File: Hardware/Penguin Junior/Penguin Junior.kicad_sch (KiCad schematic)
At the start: 30 parts, among them SW1 SW_Push, SW2 SW_SPDT, U1 STM32F405RGTx, Y1 16MHz

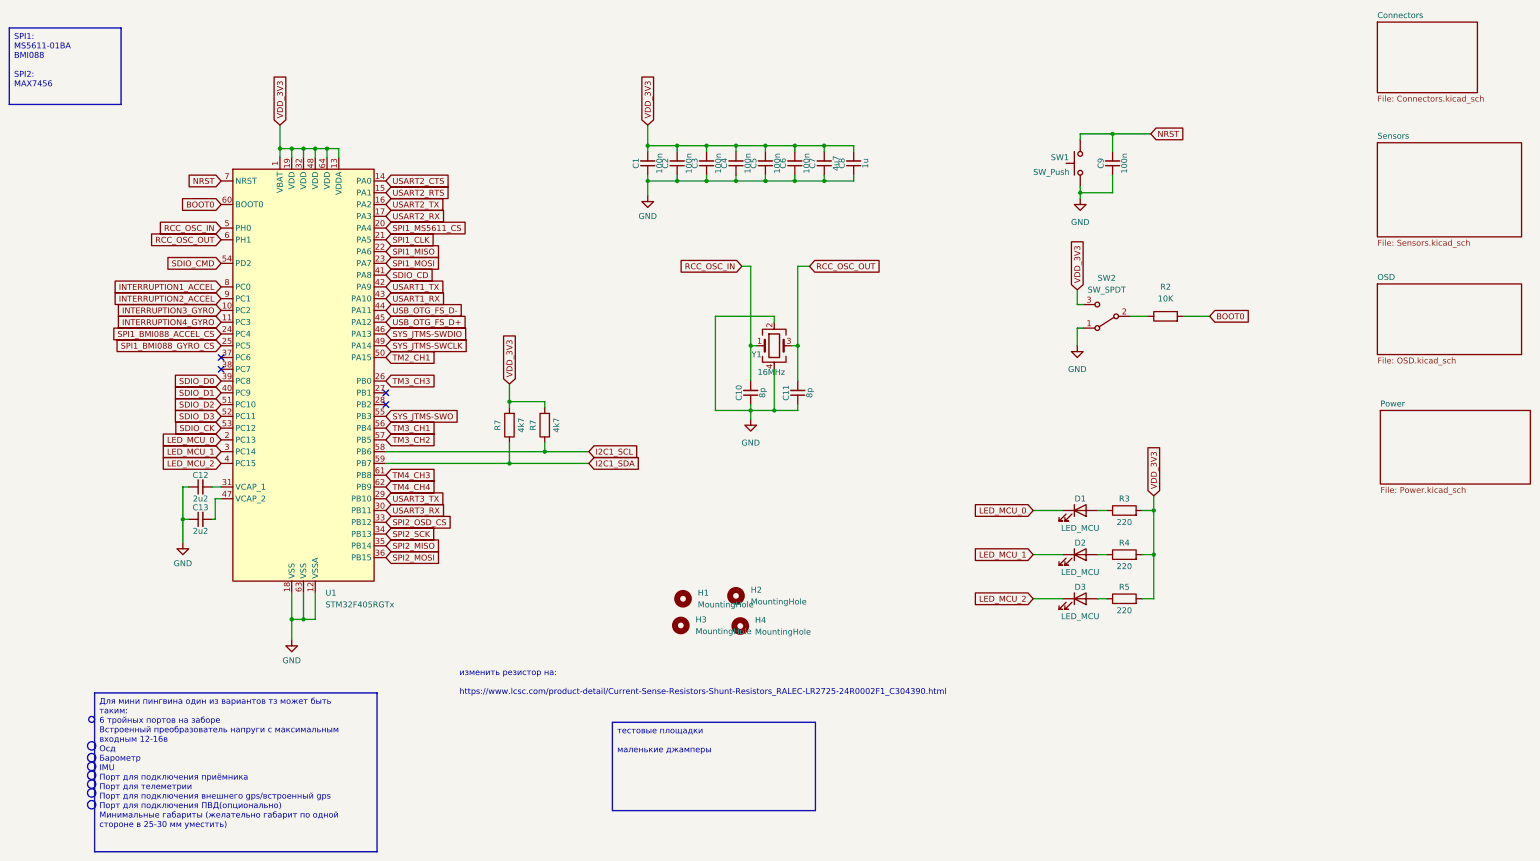
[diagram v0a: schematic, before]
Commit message: Updated project
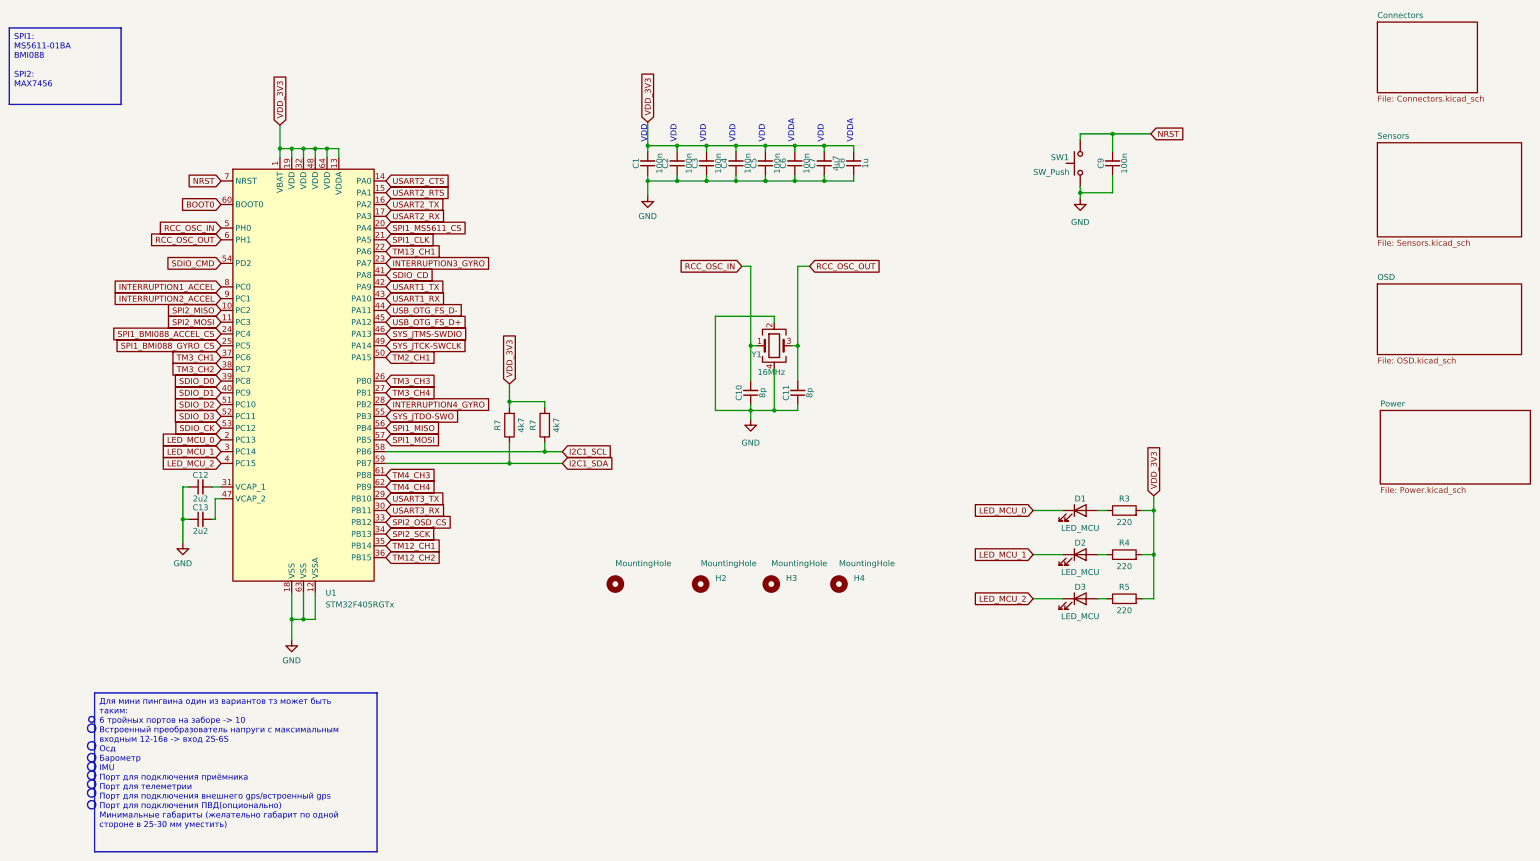
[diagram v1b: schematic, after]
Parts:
- removed R2: 10K, Resistor_SMD:R_0603_1608Metric, symbol Device:R
- removed SW2: SW_SPDT, user_lib:MSS-12D16, symbol Switch:SW_SPDT
- C1, C10, C11, C12, C13, C2, C3, C4, C5, C6, C7, C8, C9: footprint Capacitor_SMD:C_0603_1608Metric -> Capacitor_SMD:C_0402_1005Metric
- H1, H2, H3, H4: footprint user_lib:MountingHole_2.2mm_M2_Pad_Via_4.0mm -> MountingHole:MountingHole_2.2mm_M2_Pad_Via
- R3, R4, R5, R7: footprint Resistor_SMD:R_0603_1608Metric -> Resistor_SMD:R_0402_1005Metric
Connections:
- net INTERRUPTION3_GYRO: now also U1.23 (PA7); no longer U1.10 (PC2)
- net INTERRUPTION4_GYRO: now also U1.28 (PB2); no longer U1.11 (PC3)
- net SPI1_MISO: now also U1.56 (PB4); no longer U1.22 (PA6)
- net SPI1_MOSI: now also U1.57 (PB5); no longer U1.23 (PA7)
- net SPI2_MISO: now also U1.10 (PC2); no longer U1.35 (PB14)
- net SPI2_MOSI: now also U1.11 (PC3); no longer U1.36 (PB15)
- net TM3_CH1: now also U1.37 (PC6); no longer U1.56 (PB4)
- net TM3_CH2: now also U1.38 (PC7); no longer U1.57 (PB5)
- net TM3_CH4: now reaches U1.27 (PB1)
- net SYS_JTMS-SWCLK renamed SYS_JTCK-SWCLK
- net SYS_JTMS-SWO renamed SYS_JTDO-SWO
- new net TM12_CH1: U1.35 (PB14)
- new net TM12_CH2: U1.36 (PB15)
- new net TM13_CH1: U1.22 (PA6)
- no-connect marks 4 -> 0
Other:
- note added: "VDD"
- note added: "VDDA"
- note removed: "изменить резистор на: https://www.lcsc.com/product-detail/Current-Sense-Resistors-Shunt-Resistors_RALEC-LR2725-24R0002F1_C304390.html"
- moved on the sheet: H2, H3, H4

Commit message: Updated Penguin project
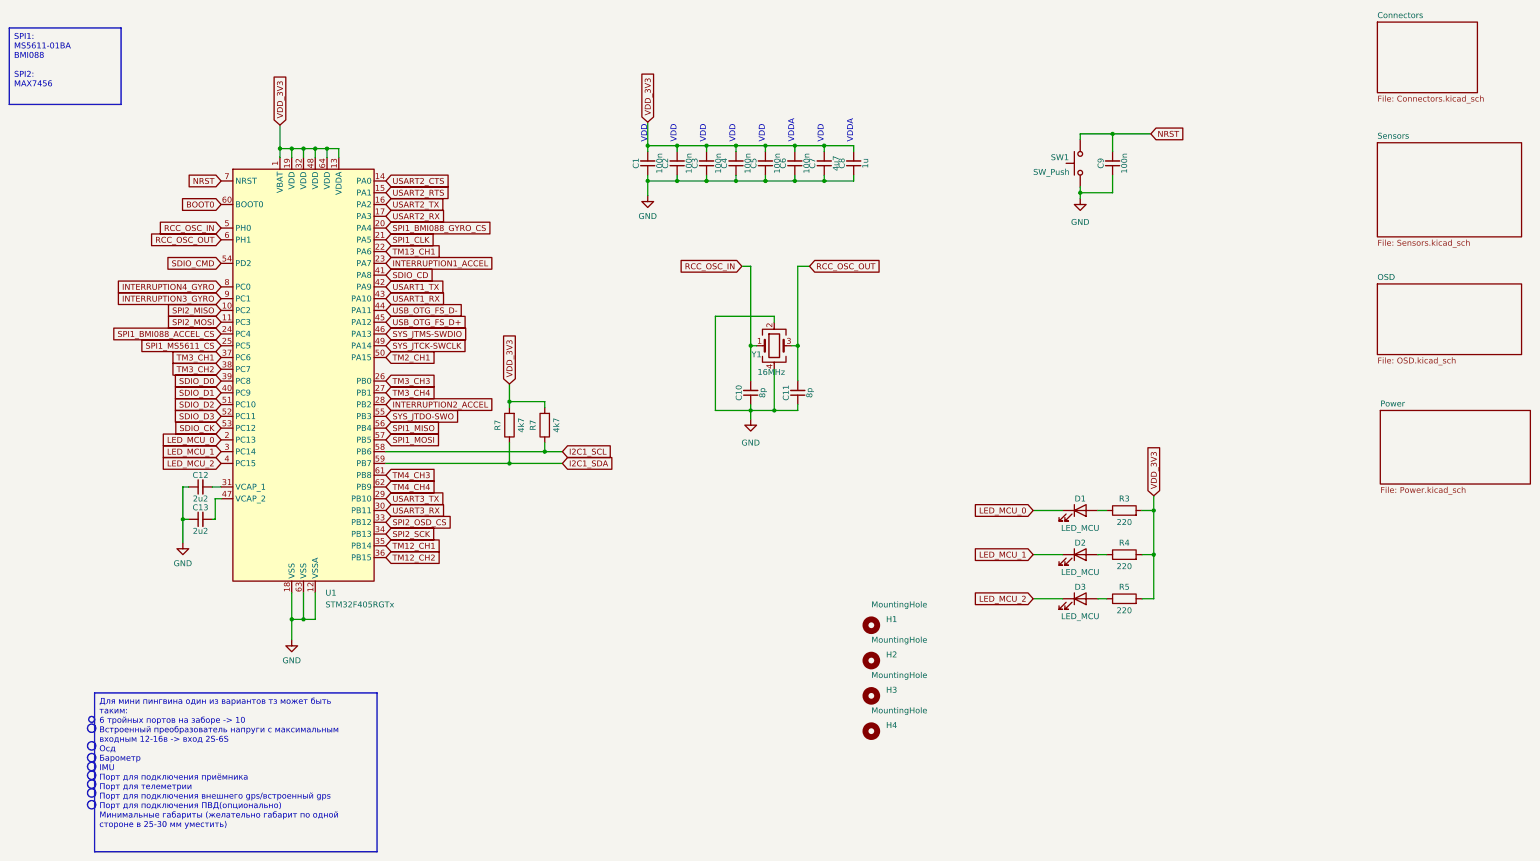
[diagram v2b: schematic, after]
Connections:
- net INTERRUPTION1_ACCEL: now also U1.23 (PA7); no longer U1.8 (PC0)
- net INTERRUPTION2_ACCEL: now also U1.28 (PB2); no longer U1.9 (PC1)
- net INTERRUPTION3_GYRO: now also U1.9 (PC1); no longer U1.23 (PA7)
- net INTERRUPTION4_GYRO: now also U1.8 (PC0); no longer U1.28 (PB2)
- net SPI1_BMI088_GYRO_CS: now also U1.20 (PA4); no longer U1.25 (PC5)
- net SPI1_MS5611_CS: now also U1.25 (PC5); no longer U1.20 (PA4)
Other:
- moved on the sheet: H2, H3, H4

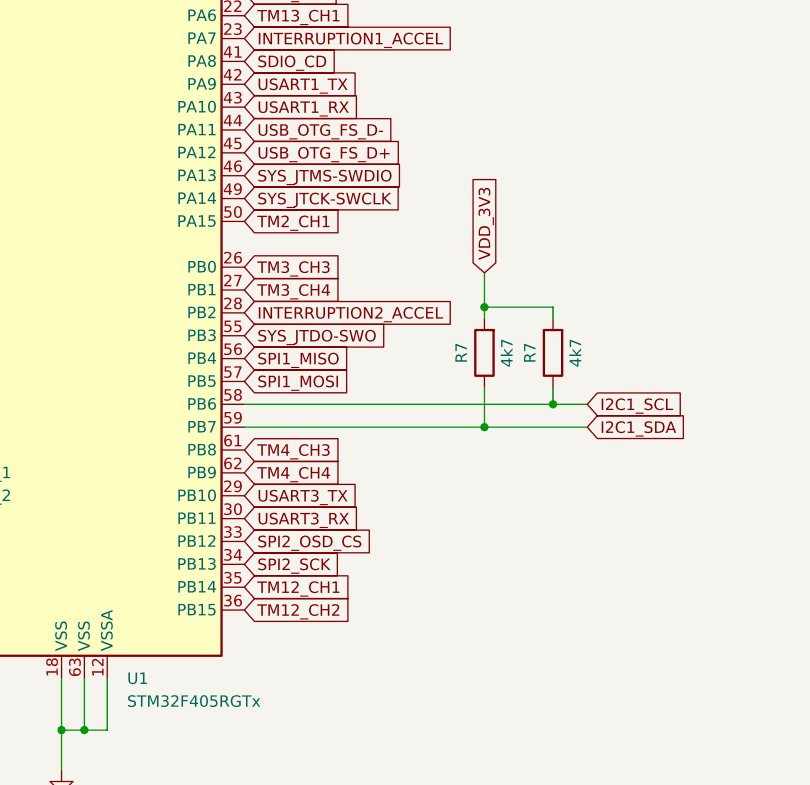
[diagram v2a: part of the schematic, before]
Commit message: Updated Penguin project
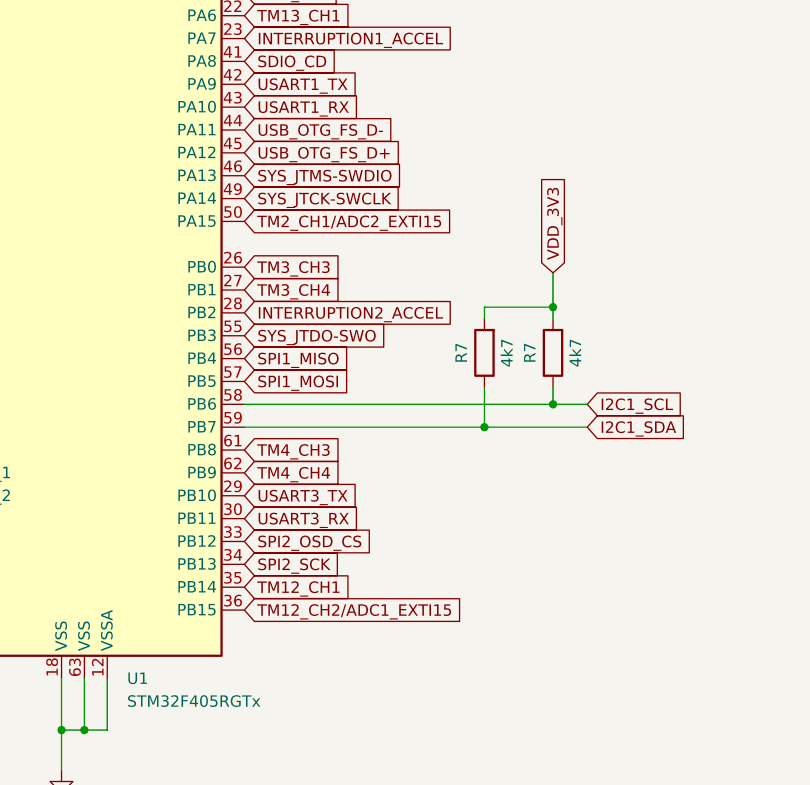
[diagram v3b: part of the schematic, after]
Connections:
- net TM12_CH2 renamed TM12_CH2/ADC1_EXTI15
- net TM2_CH1 renamed TM2_CH1/ADC2_EXTI15
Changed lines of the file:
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@@
   (junction (at 241.3 46.99) (diameter 0) (color 0 0 0 0)
   )
-  (junction (at 118.11 92.075) (diameter 0) (color 0 0 0 0)
-  )
   (junction (at 118.11 105.41) (diameter 0) (color 0 0 0 0)
   )
@@
   (junction (at 173.355 36.83) (diameter 0) (color 0 0 0 0)
   )
+  (junction (at 125.73 92.075) (diameter 0) (color 0 0 0 0)
+  )
   (junction (at 186.055 36.83) (diameter 0) (color 0 0 0 0)
   )
@@
     (stroke (width 0) (type default))
   )
-  (wire (pts (xy 118.11 88.265) (xy 118.11 92.075))
+  (wire (pts (xy 125.73 88.265) (xy 125.73 92.075))
     (stroke (width 0) (type default))
   )
@@
     (stroke (width 0) (type default))
   )
-  (wire (pts (xy 118.11 92.075) (xy 125.73 92.075))
-    (stroke (width 0) (type default))
-  )
   (wire (pts (xy 76.2 37.465) (xy 76.2 39.37))
     (stroke (width 0) (type default))
@@
   )
   (wire (pts (xy 170.18 80.01) (xy 171.45 80.01))
+    (stroke (width 0) (type default))
+  )
+  (wire (pts (xy 125.73 92.075) (xy 118.11 92.075))
     (stroke (width 0) (type default))
   )
@@
     )
   )
+  (global_label "TM12_CH2{slash}ADC1_EXTI15" (shape input) (at 91.44 125.73 0) (fields_autoplaced)
+    (effects (font (size 1.27 1.27)) (justify left))
+    (property "Intersheetrefs" "${INTERSHEET_REFS}" (at 117.5269 125.73 0)
+      (effects (font (size 1.27 1.27)) (justify left) hide)
+    )
+  )
   (global_label "TM3_CH4" (shape input) (at 91.44 90.17 0) (fields_autoplaced)
     (effects (font (size 1.27 1.27)) (justify left))
@@
     )
   )
-  (global_label "TM12_CH2" (shape input) (at 91.44 125.73 0) (fields_autoplaced)
-    (effects (font (size 1.27 1.27)) (justify left))
-    (property "Intersheetrefs" "${INTERSHEET_REFS}" (at 104.0408 125.73 0)
-      (effects (font (size 1.27 1.27)) (justify left) hide)
-    )
-  )
   (global_label "INTERRUPTION3_GYRO" (shape input) (at 55.88 69.85 180) (fields_autoplaced)
     (effects (font (size 1.27 1.27)) (justify right))
@@
     )
   )
-  (global_label "TM2_CH1" (shape input) (at 91.44 82.55 0) (fields_autoplaced)
-    (effects (font (size 1.27 1.27)) (justify left))
-    (property "Intersheetrefs" "${INTERSHEET_REFS}" (at 102.8313 82.55 0)
-      (effects (font (size 1.27 1.27)) (justify left) hide)
-    )
-  )
   (global_label "INTERRUPTION4_GYRO" (shape input) (at 55.88 67.31 180) (fields_autoplaced)
     (effects (font (size 1.27 1.27)) (justify right))
@@
     )
   )
-  (global_label "VDD_3V3" (shape input) (at 118.11 88.265 90) (fields_autoplaced)
-    (effects (font (size 1.27 1.27)) (justify left))
-    (property "Intersheetrefs" "${INTERSHEET_REFS}" (at 118.11 77.176 90)
+  (global_label "VDD_3V3" (shape input) (at 125.73 88.265 90) (fields_autoplaced)
+    (effects (font (size 1.27 1.27)) (justify left))
+    (property "Intersheetrefs" "${INTERSHEET_REFS}" (at 125.73 77.176 90)
       (effects (font (size 1.27 1.27)) (justify left) hide)
     )
@@
       (effects (font (size 1.27 1.27)) (justify left) hide)
     )
+  )
+  (global_label "TM2_CH1{slash}ADC2_EXTI15" (shape input) (at 91.44 82.55 0) (fields_autoplaced)
+    (effects (font (size 1.27 1.27)) (justify left))
+    (property "Intersheetrefs" "${INTERSHEET_REFS}" (at 116.3174 82.55 0)
+      (effects (font (size 1.27 1.27)) (justify left) hide)
+    )
